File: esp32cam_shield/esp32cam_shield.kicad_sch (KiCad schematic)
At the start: 52 parts, among them J1 ESP32 CAM, J2 Battery, J3 Motor, J4 Motor, J5 Motor, J6 Motor, Q1 NMOS, Q2 NMOS, Q3 NMOS, Q4 NMOS, U1 MPU-6050, U2 LMR62421XMF

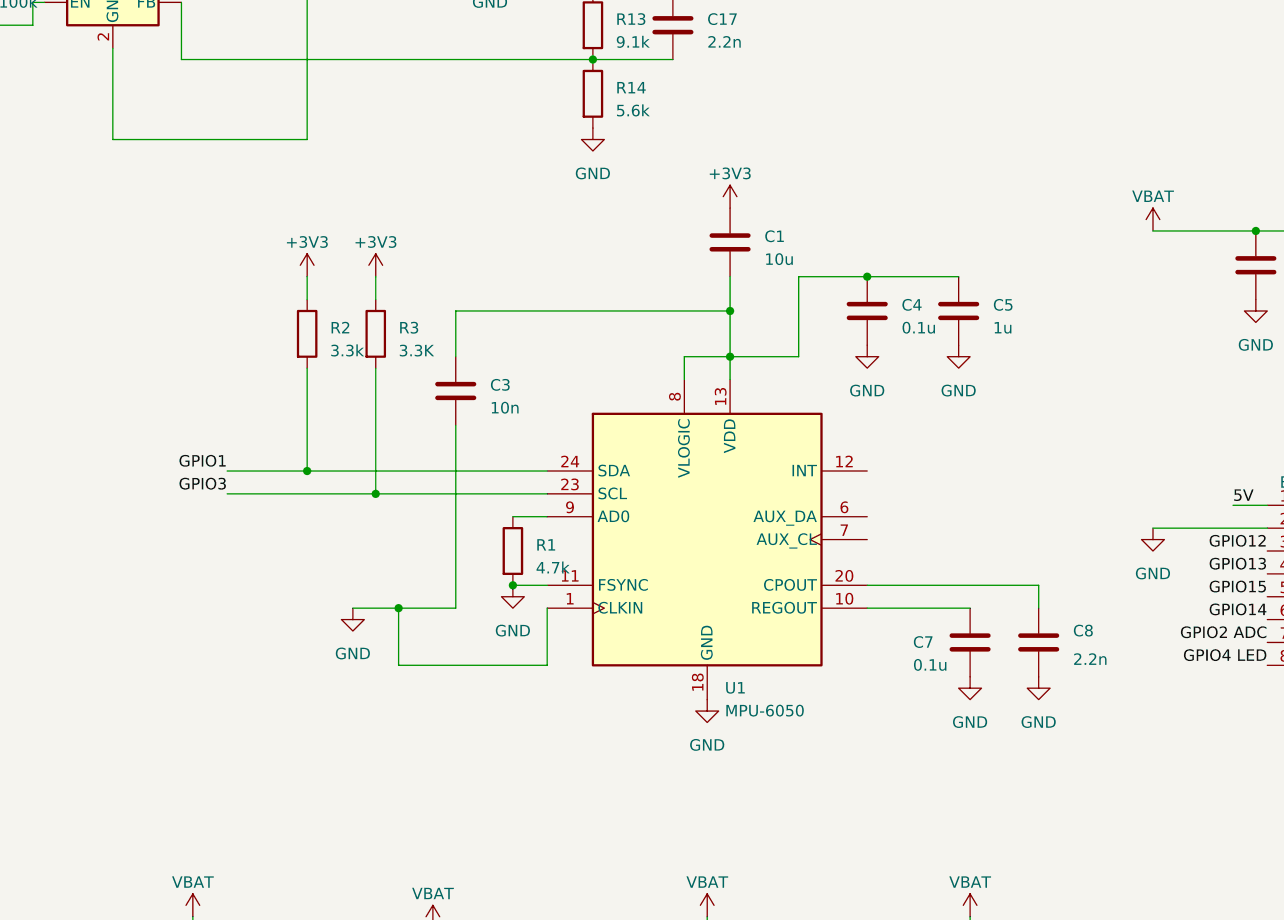
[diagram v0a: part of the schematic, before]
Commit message: MPU-6050 modul
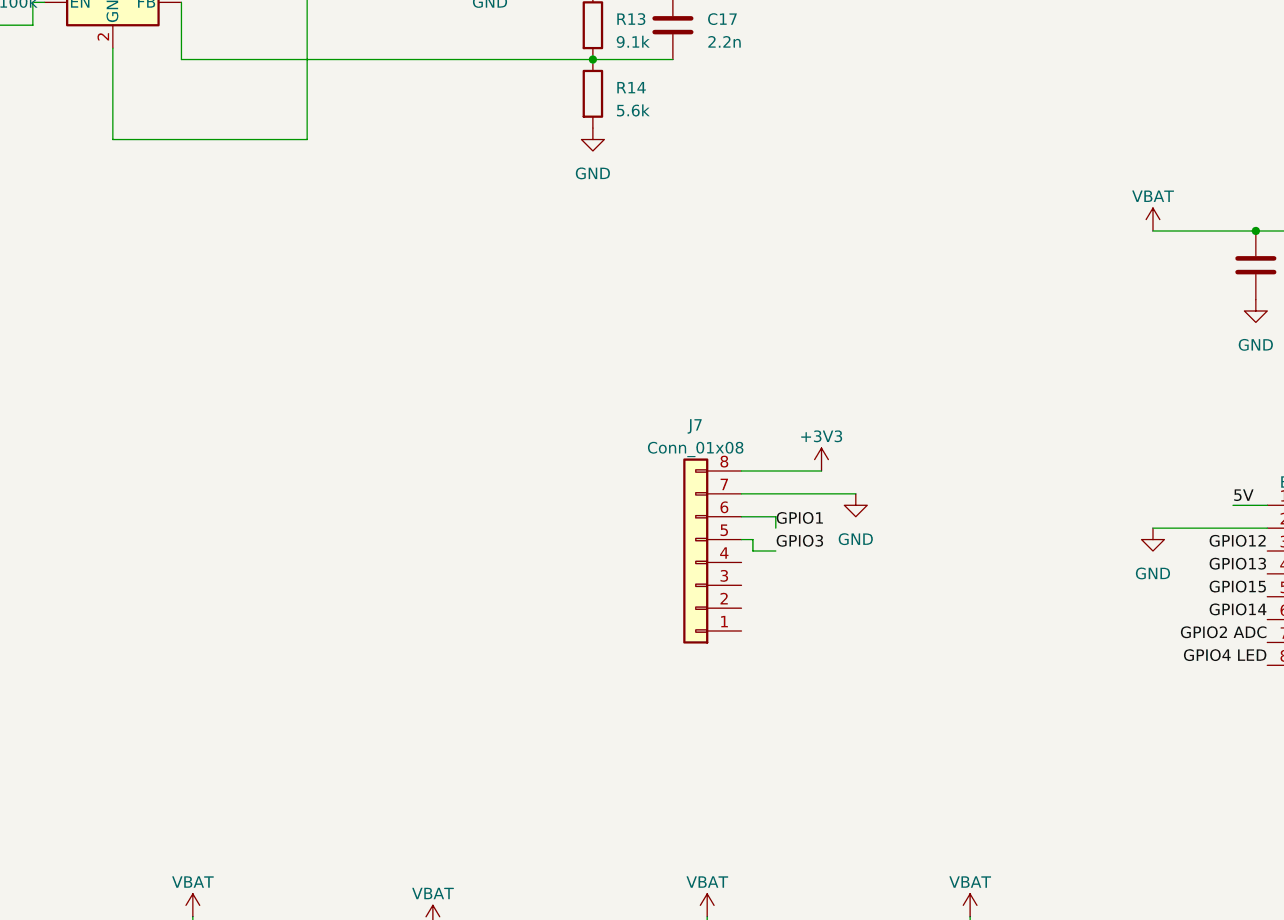
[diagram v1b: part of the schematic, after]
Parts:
- removed C1: 10u, Capacitor_SMD:C_1206_3216Metric_Pad1.33x1.80mm_HandSolder, symbol Device:C
- removed C3: 10n, Capacitor_SMD:C_0805_2012Metric_Pad1.18x1.45mm_HandSolder, symbol Device:C
- removed C4, C7: 0.1u, Capacitor_SMD:C_0805_2012Metric_Pad1.18x1.45mm_HandSolder, symbol Device:C
- removed C5: 1u, Capacitor_SMD:C_0805_2012Metric_Pad1.18x1.45mm_HandSolder, symbol Device:C
- removed C8: 2.2n, Capacitor_SMD:C_0805_2012Metric_Pad1.18x1.45mm_HandSolder, symbol Device:C
- removed R1: 4.7k, Resistor_SMD:R_0805_2012Metric_Pad1.20x1.40mm_HandSolder, symbol Device:R
- removed R2: 3.3k, Resistor_SMD:R_0805_2012Metric_Pad1.20x1.40mm_HandSolder, symbol Device:R
- removed R3: 3.3K, Resistor_SMD:R_0805_2012Metric_Pad1.20x1.40mm_HandSolder, symbol Device:R
- removed U1: MPU-6050, Sensor_Motion:InvenSense_QFN-24_4x4mm_P0.5mm, symbol Sensor_Motion:MPU-6050
- added J7: Conn_01x08, Connector_PinSocket_2.54mm:PinSocket_1x08_P2.54mm_Vertical, symbol Connector_Generic:Conn_01x08
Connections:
- net +3V3: now also J7.8 (Pin_8)
- net GND: now also J7.7 (Pin_7)
- net GPIO1: now also J7.6 (Pin_6)
- net GPIO3: now also J7.5 (Pin_5)
